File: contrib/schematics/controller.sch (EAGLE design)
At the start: 31 parts, among them IC2 MAX 603, IC3 MEGA16-P, Q1 16 MHz, T1 BS-107, T2 BS-107

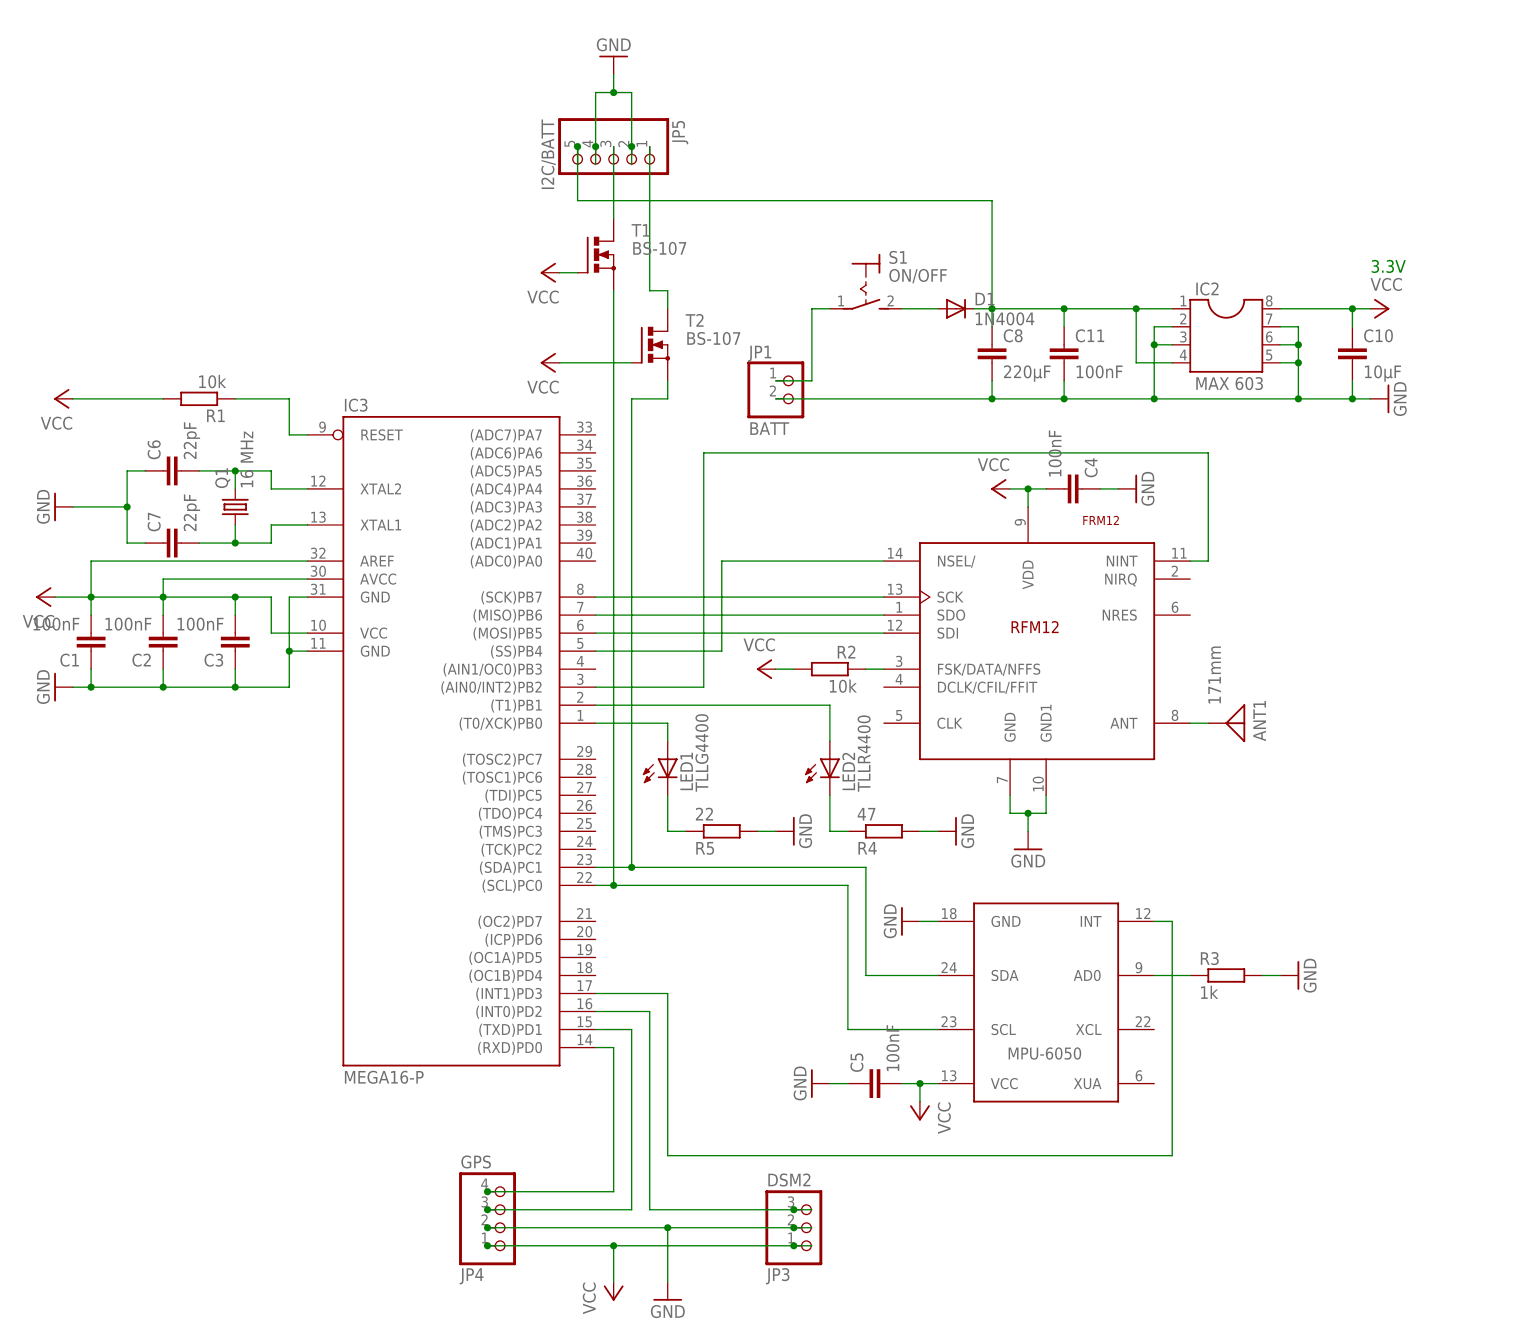
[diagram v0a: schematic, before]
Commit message: Updated controller board
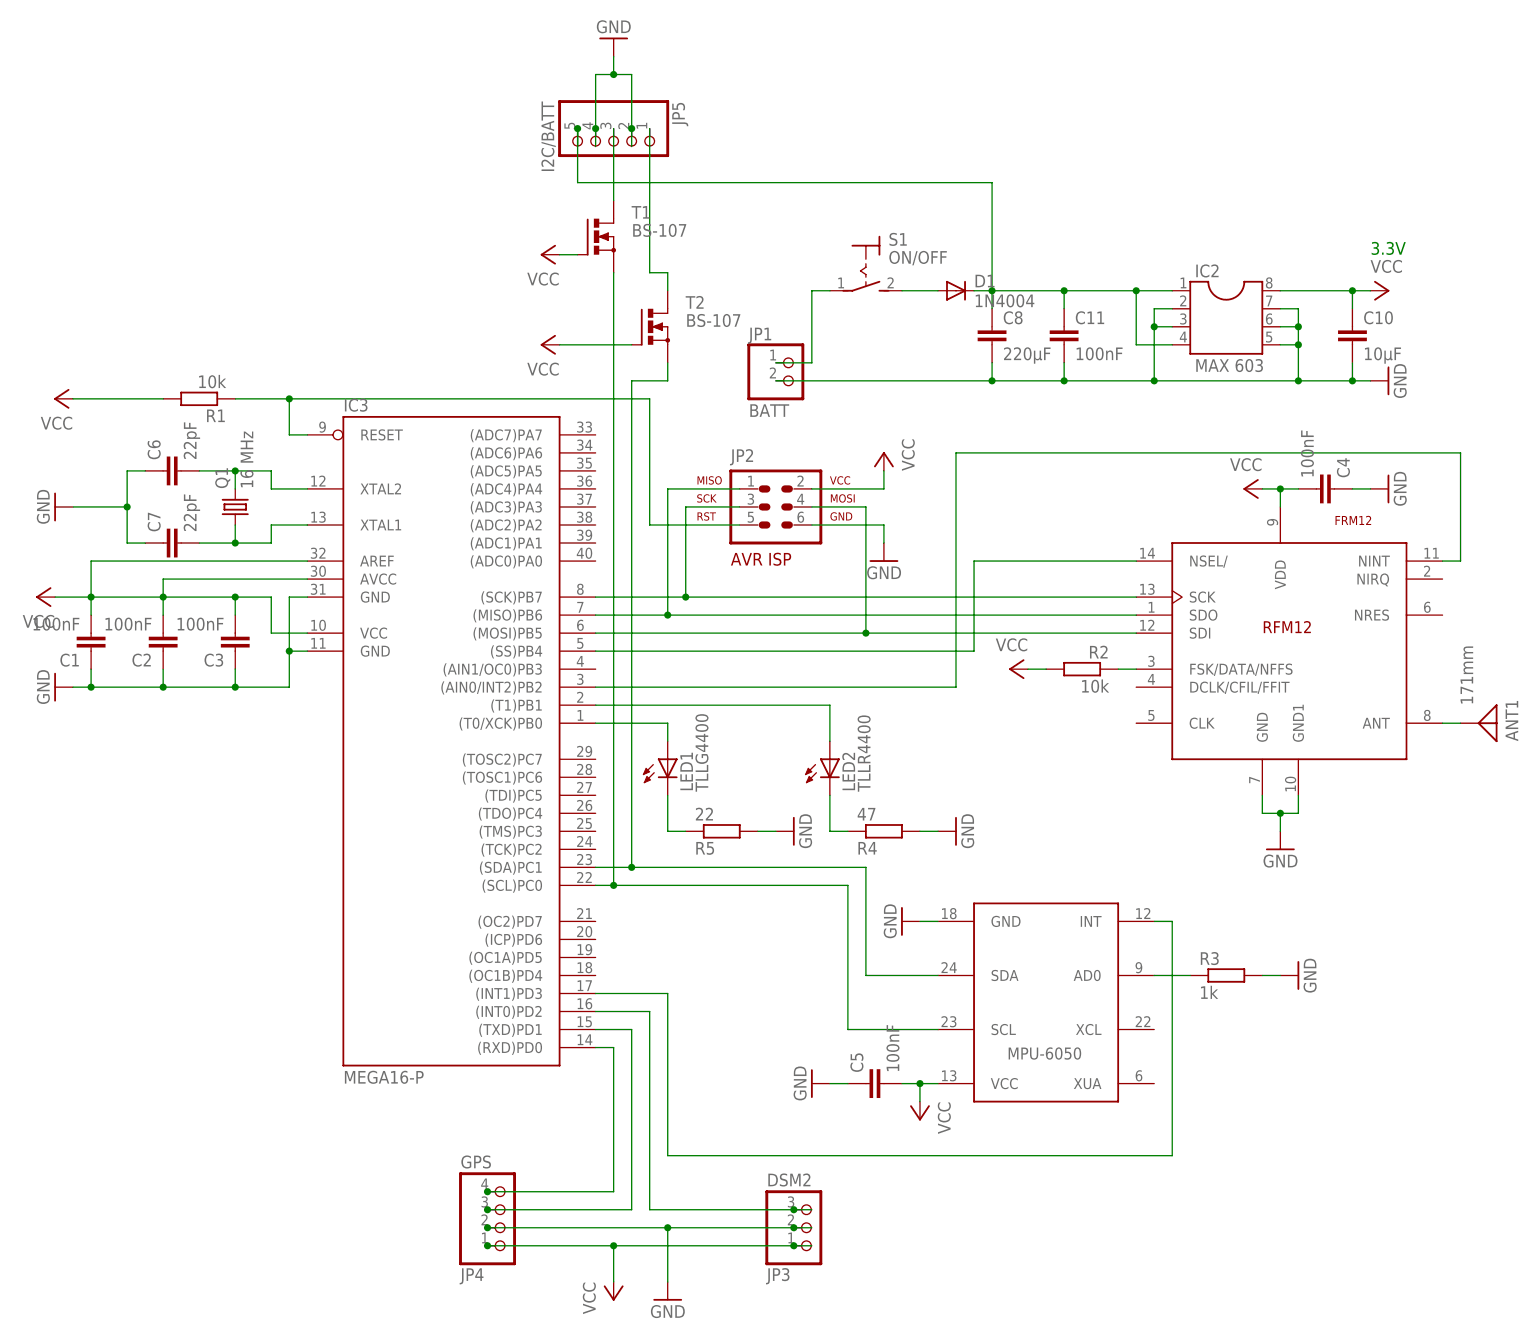
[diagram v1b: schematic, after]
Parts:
- added JP2: AVR-ISP-6VERT, avr-7:AVR-ISP-6VERT
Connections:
- net GND: now also JP2.6
- net N$12: now also JP2.4
- net N$14: now also JP2.1
- net N$15: now also JP2.3
- net N$24: now also C11.1
- net N$9: now also JP2.5
- net VCC: now also JP2.2
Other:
- moved on the sheet: ANT1, C10, C11, C4, C8, D1, IC2, JP1, JP5, R2, S1, T1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
